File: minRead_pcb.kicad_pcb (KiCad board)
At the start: 2 copper layers, 133.9 x 116.2 mm, 121 parts, among them J1 USB_C_Receptacle, J2 FH34SRJ-24S-0.5SH_50_, J3 FH34SRJ-6S-0.5SH_50_, J5 Conn_01x02, J7 Micro_SD_Card, Q10 BSS138, Q11 BSS138, Q16 MMBT3906, Q17 MMBT3904, Q18 AO3419, Q4 [BSS138] AO3400A, Q5 AO3419, SW1 SW_Push, SW10 SW_Push, SW11 SW_Push, SW2 SW_Push, SW3 SW_Push, SW4 SW_Push, SW6 SW_Push, SW8 SW_Push, SW9 SW_Push, U1 TPD4E1U06DBVR, U11 AP3031KTR, U2 TPS2116DRL, U3 AP2112K-3.3, U4 ESP32-S3-WROOM-1, U6 TPD4E1U06DBVR, U7 MCP73832-2-OT

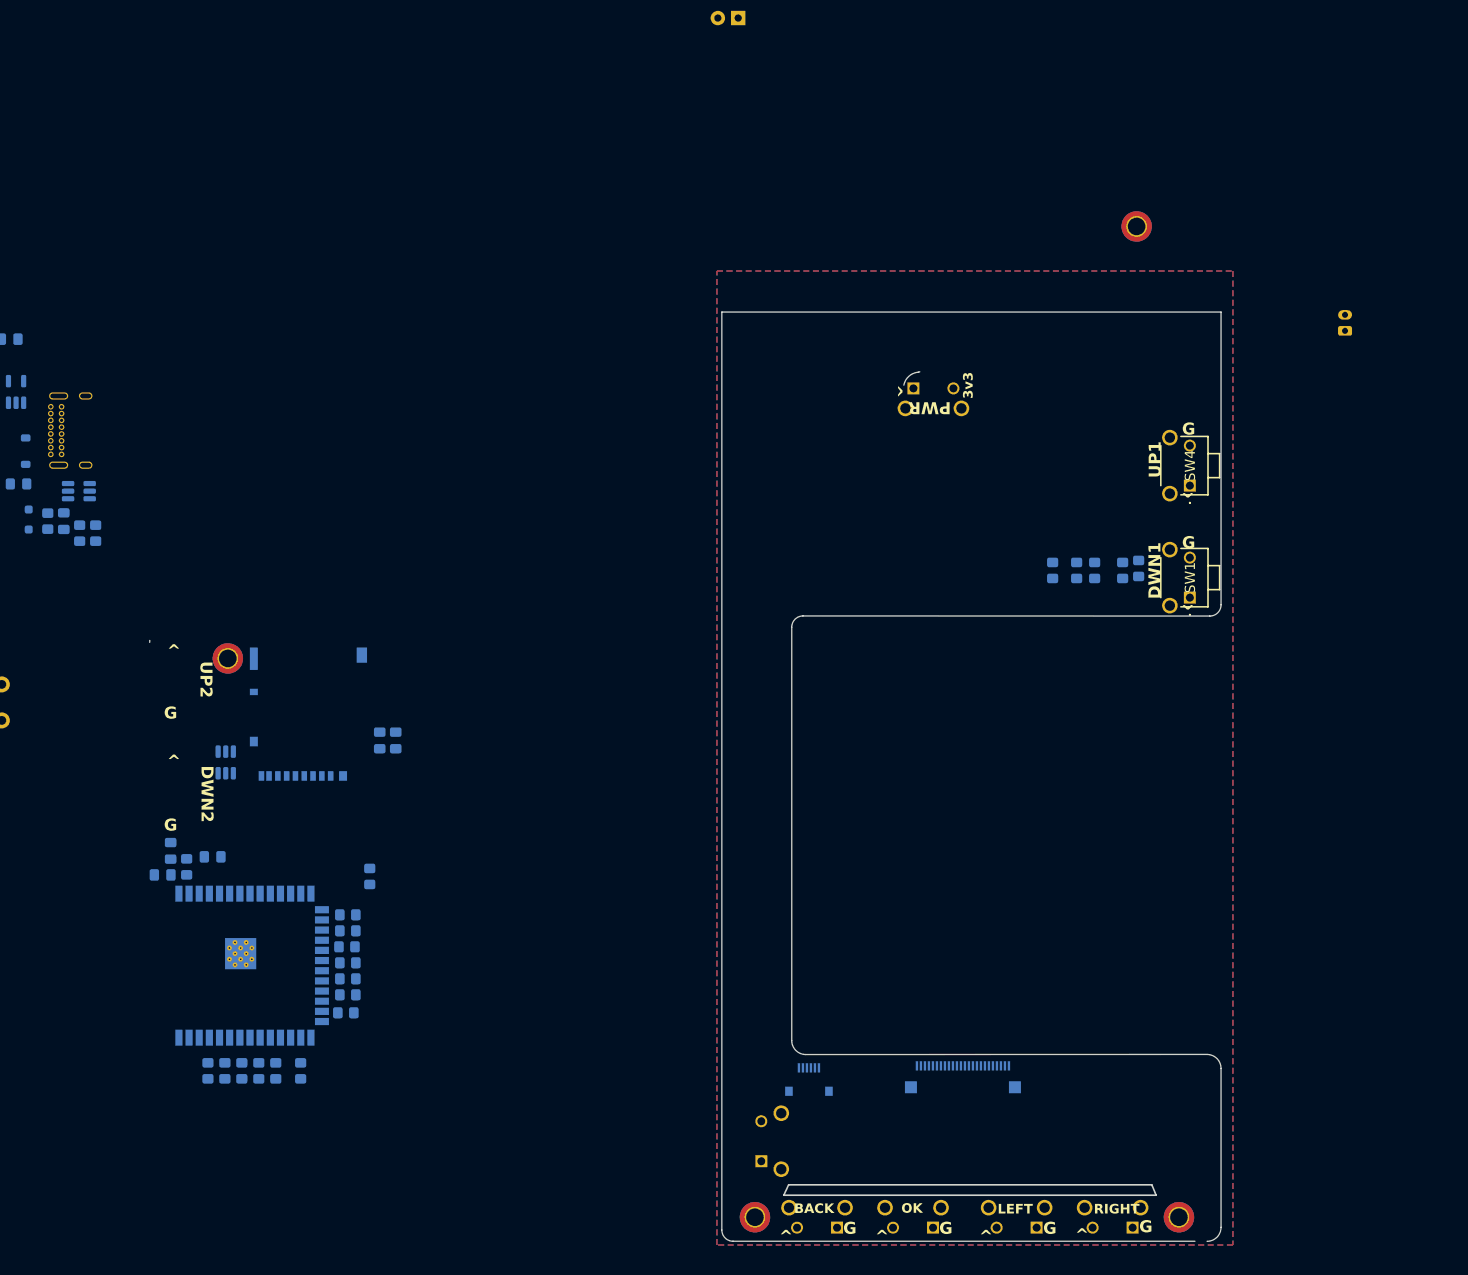
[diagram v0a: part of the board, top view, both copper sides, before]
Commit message: general setup prep for routing
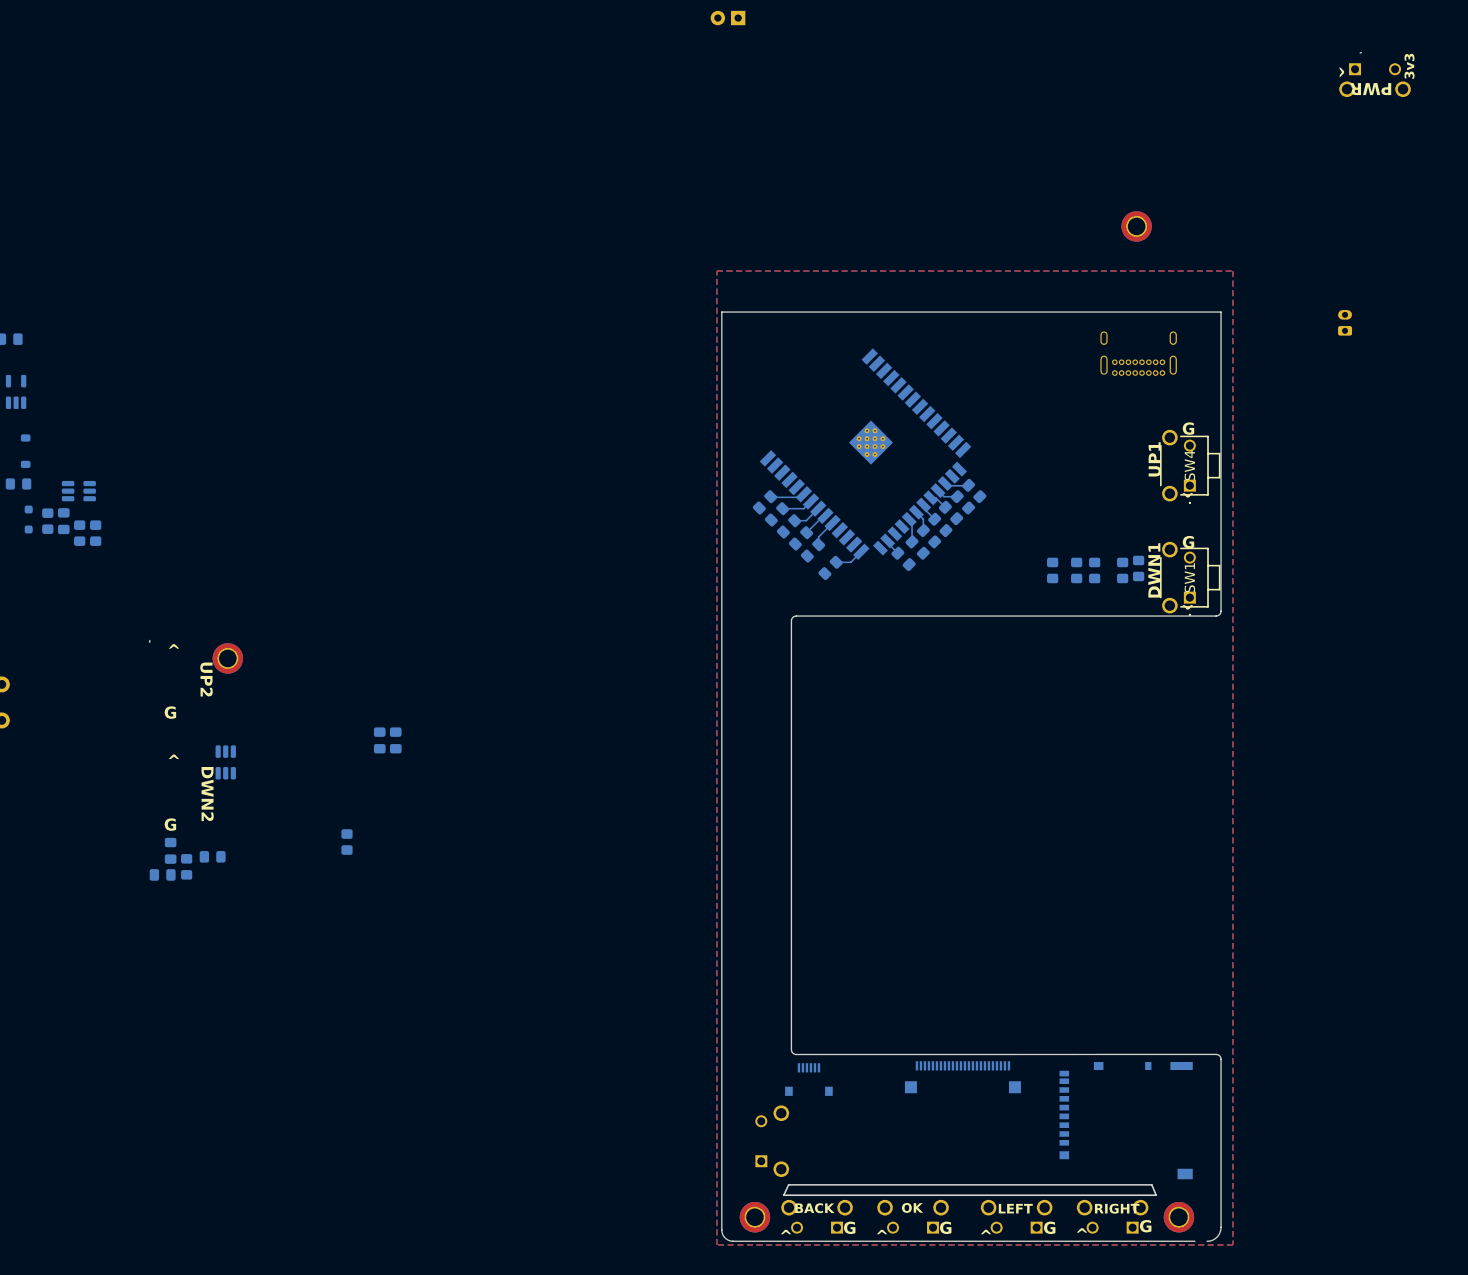
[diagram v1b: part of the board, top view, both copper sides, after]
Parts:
- moved J1 133.1 mm to (92.5, 39.7), turned to 0 degrees
- moved J7 114.1 mm to (93.9, 133.2), turned to -90 degrees
- moved U4 102.6 mm to (59.2, 47.7), turned to -135 degrees
- moved R21 99.5 mm to (48.7, 55.9), turned to -135 degrees
- moved R22 98.0 mm to (50.2, 57.4), turned to -135 degrees
- moved R23 96.5 mm to (51.7, 58.9), turned to -135 degrees
- moved R25 95.0 mm to (53.2, 60.4), turned to -135 degrees
- moved R29 94.5 mm to (74.9, 54.5), turned to 135 degrees
- moved R30 93.7 mm to (73.5, 55.9), turned to 135 degrees
- moved R24 93.5 mm to (54.7, 61.9), turned to -135 degrees
- moved R31 93.0 mm to (72.0, 57.2), turned to 135 degrees
- moved R32 92.1 mm to (70.7, 58.7), turned to 135 degrees
- moved R13 91.3 mm to (56.9, 64.1), turned to 45 degrees
- moved R33 91.3 mm to (69.2, 60.1), turned to 135 degrees
- moved R34 90.6 mm to (67.8, 61.5), turned to 135 degrees
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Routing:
- net Net-(U4-IO42): track 0.00 -> 4.34 mm
- net Net-(U4-IO41): track 0.00 -> 3.93 mm
- net ESP32_IO0: track 0.00 -> 3.68 mm
- net Net-(U4-IO40): track 0.00 -> 3.57 mm
- net Net-(U4-IO38): track 0.00 -> 3.43 mm
- net Net-(U4-IO39): track 0.00 -> 3.22 mm
- net Net-(U4-IO9): track 0.00 -> 3.07 mm
- net Net-(U4-IO14): track 0.00 -> 2.96 mm
- net Net-(U4-IO10): track 0.00 -> 2.72 mm
- net Net-(U4-IO13): track 0.00 -> 2.66 mm
- net Net-(U4-IO12): track 0.00 -> 2.35 mm
- net Net-(U4-IO11): track 0.00 -> 2.31 mm
- net Net-(U4-IO48): track 0.00 -> 2.06 mm
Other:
- board size 133.9 x 116.2 mm -> 151.5 x 148.6 mm
